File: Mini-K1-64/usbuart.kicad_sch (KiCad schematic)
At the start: 12 parts, among them P1 USB_C_Plug_USB2.0, U1 CH343G, U3 AMS1117-3.3

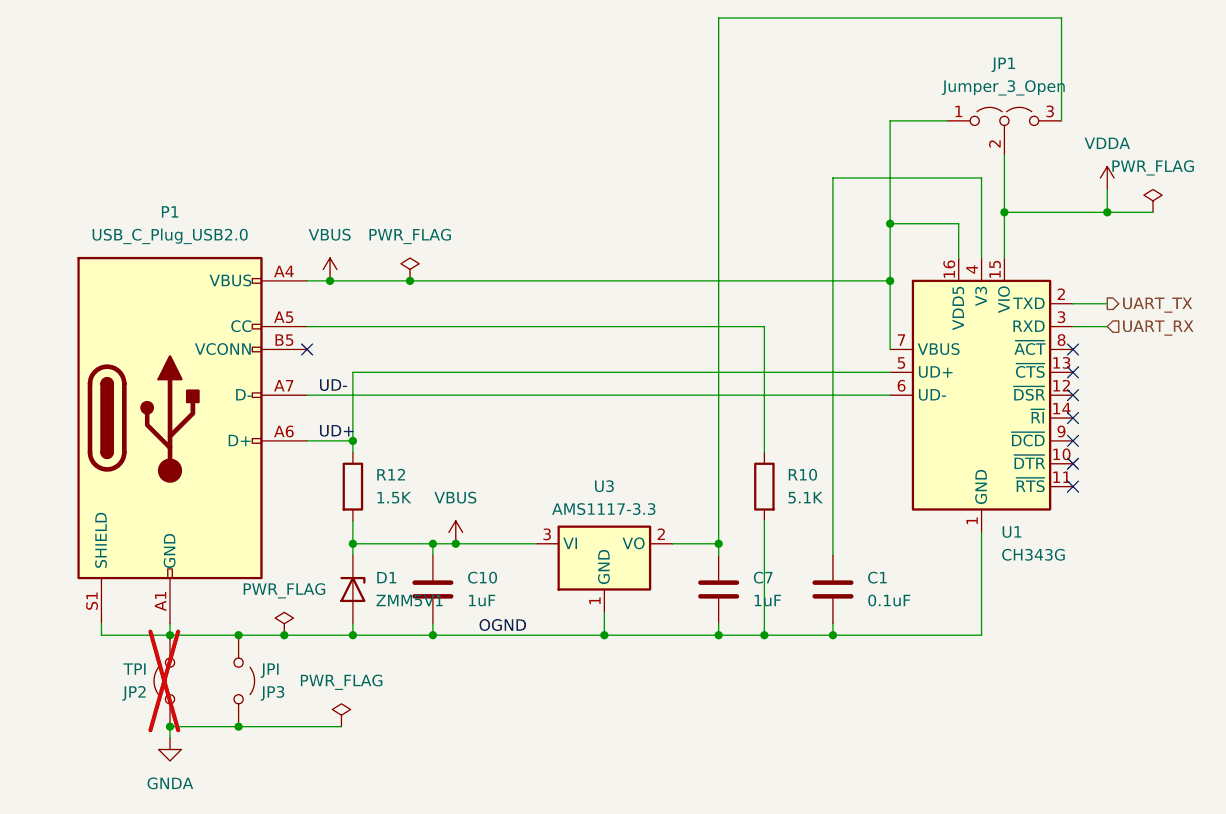
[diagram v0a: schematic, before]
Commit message: Step Update
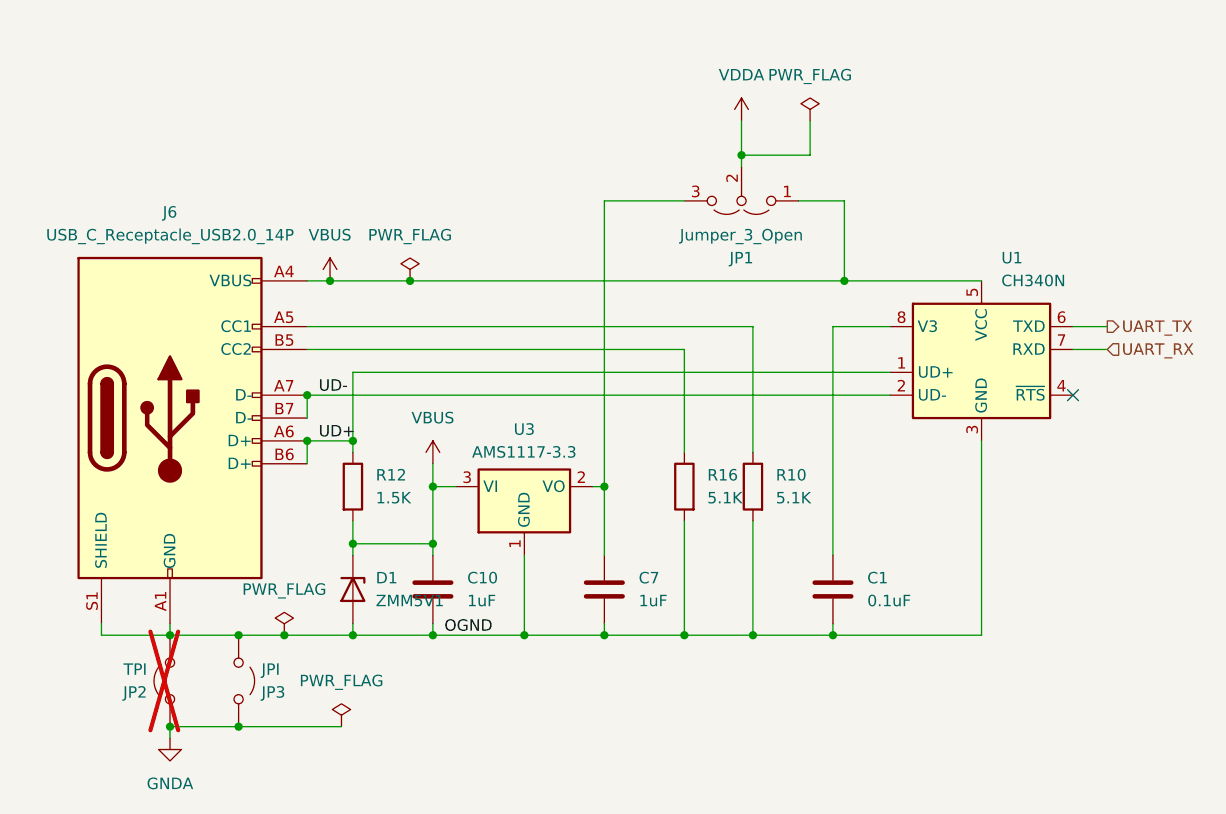
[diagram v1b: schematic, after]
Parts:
- removed P1: USB_C_Plug_USB2.0, Connector_USB:USB_C_Receptacle_GCT_USB4105-xx-A_16P_TopMnt_Horizontal, symbol Connector:USB_C_Plug_USB2.0
- removed U1: CH343G, Package_SO:SOIC-16_3.9x9.9mm_P1.27mm, symbol Interface_USB:CH343G
- added J6: USB_C_Receptacle_USB2.0_14P, Connector_USB:USB_C_Receptacle_GCT_USB4105-xx-A_16P_TopMnt_Horizontal, symbol Connector:USB_C_Receptacle_USB2.0_14P
- added R16: 5.1K, Resistor_SMD:R_0805_2012Metric, symbol Device:R
- added U1: CH340N, Package_SO:SOP-8_3.9x4.9mm_P1.27mm, symbol Interface_USB:CH340N
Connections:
- net OGND: now also J6.A1 (GND), J6.A12 (GND), J6.B1 (GND), J6.B12 (GND), J6.S1 (SHIELD), R16.2, U1.3 (GND)
- net UART_RX: now also U1.7 (RXD)
- net UART_TX: now also U1.6 (TXD)
- net UD+: now also J6.A6 (D+), J6.B6 (D+), U1.1 (UD+)
- net UD-: now also J6.A7 (D-), J6.B7 (D-), U1.2 (UD-)
- net VBUS: now also J6.A4 (VBUS), J6.A9 (VBUS), J6.B4 (VBUS), J6.B9 (VBUS), U1.5 (VCC)
- net at C1.1: now also U1.8 (V3)
- net at R10.1: now also J6.A5 (CC1)
- new net: J6.B5 (CC2), R16.1
- no-connect marks 8 -> 1
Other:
- moved on the sheet: C7, R10, U3
